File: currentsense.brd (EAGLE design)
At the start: 78.7 x 70.8 mm, 18 parts

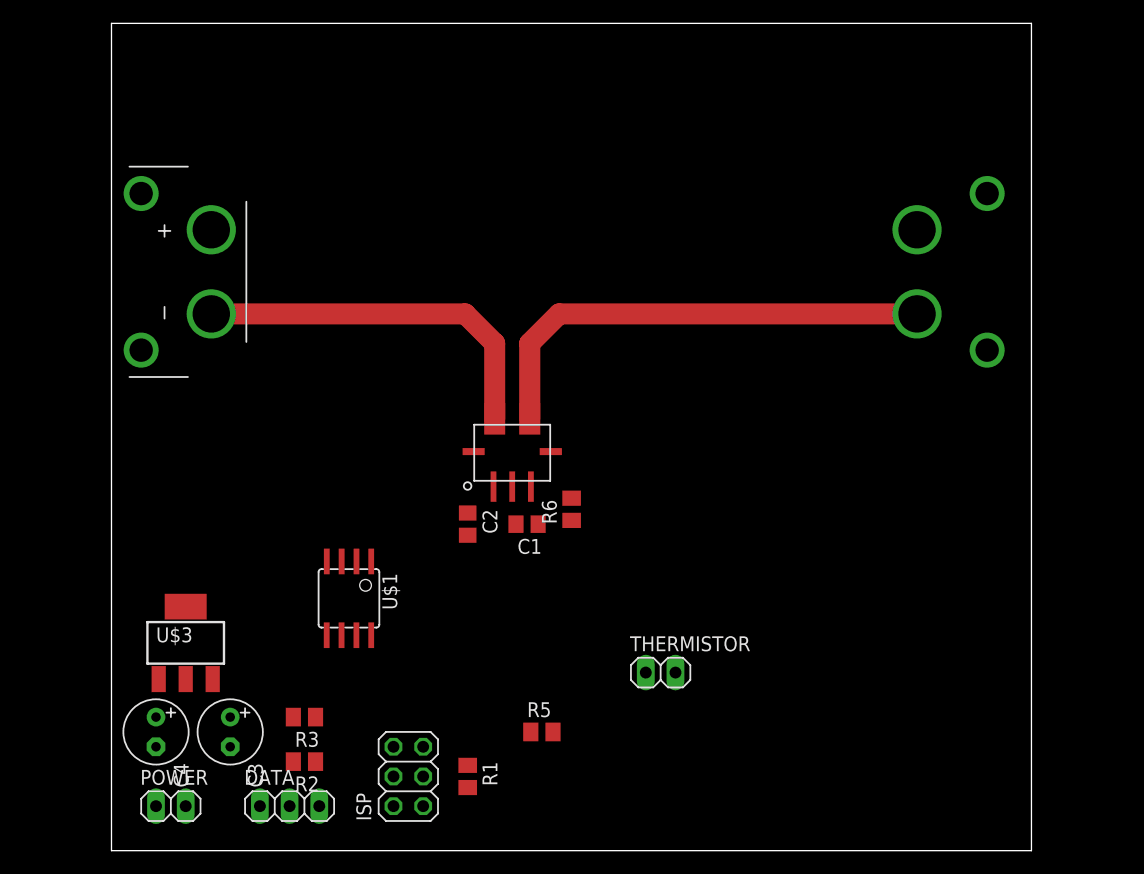
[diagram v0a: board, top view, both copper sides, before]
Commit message: more layout work
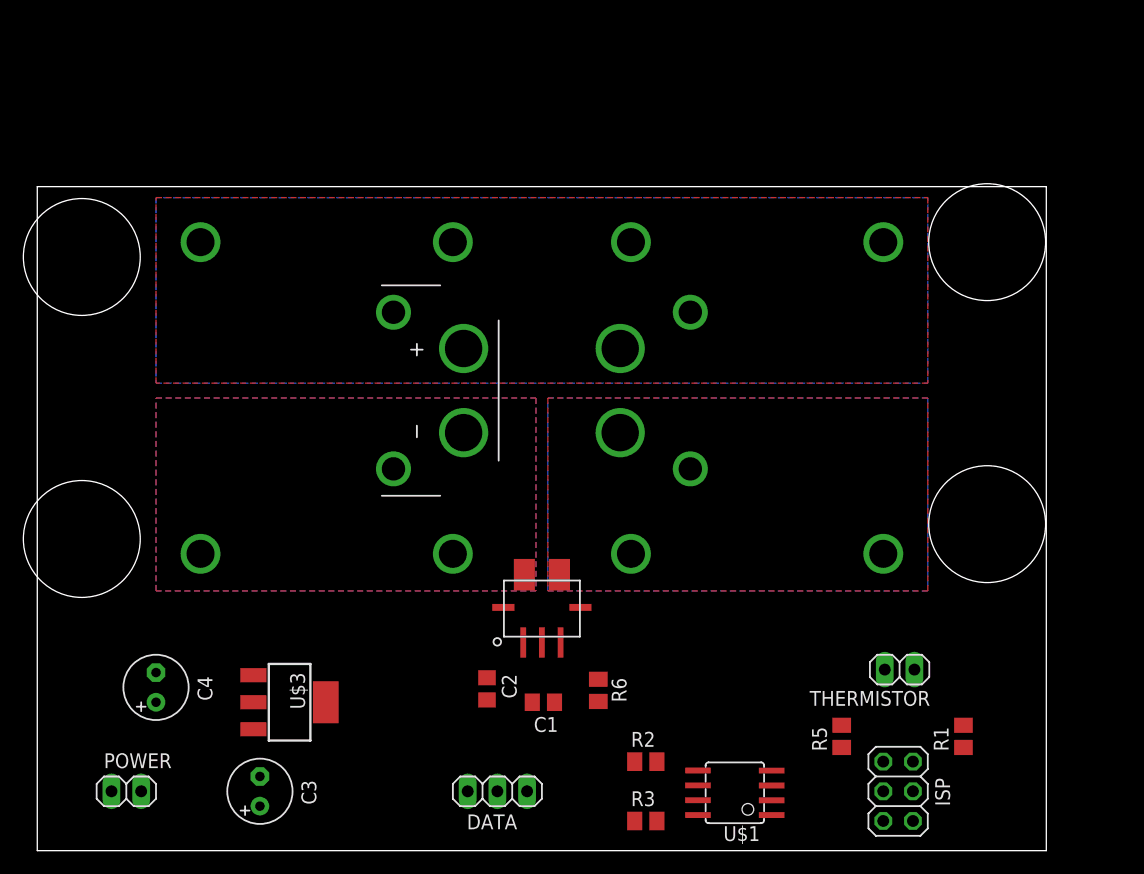
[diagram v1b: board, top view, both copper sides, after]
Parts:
- moved R1 42.6 mm to (72.9, 9.78), turned to 90 degrees
- moved ISP 41.9 mm to (67.3, 5.08)
- moved U$1 37.0 mm to (53.3, 4.95), turned to 90 degrees
- moved R3 30.5 mm to (45.7, 2.54), turned to 0 degrees
- moved R2 29.2 mm to (45.7, 7.62), turned to 0 degrees
- moved U$4 27.4 mm to (49.5, 39.4)
- moved R5 25.7 mm to (62.5, 9.78), turned to 90 degrees
- moved U$5 23.9 mm to (24.1, 39.4)
- moved THERMISTOR 20.4 mm to (67.4, 15.5), turned to 180 degrees
- moved DATA 17.8 mm to (33.0, 5.08)
- moved R6 15.7 mm to (41.7, 13.7)
- moved C1 15.3 mm to (37.0, 12.7)
- moved C2 14.2 mm to (32.1, 13.8)
- moved U$2 13.6 mm to (36.8, 18.4)
- moved U$3 10.2 mm to (15.2, 12.7), turned to 270 degrees
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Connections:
- net N$1 renamed M-IP+
- net N$3 renamed M-IP-
- net N$4 renamed M+
- removed net OC_DETECT: DATA.3
- removed net SDA: DATA.1
- net OC_DETECT/6: now also DATA.2
- net SCL/7: now also DATA.3; no longer DATA.2
- net SDA/5: now also DATA.1
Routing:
- net M-IP+: track 40.6 -> 0.00 mm, vias 0 -> 2
- net M-IP-: track 31.8 -> 0.00 mm, vias 0 -> 2
- added copper zone on layer 1, net M+
- added copper zone on layer 16, net M+
- added copper zone on layer 1, net M-IP+
- added copper zone on layer 16, net M-IP+
- added copper zone on layer 1, net M-IP-
- added copper zone on layer 16, net M-IP-
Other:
- board size 78.7 x 70.8 mm -> 86.3 x 56.8 mm

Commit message: add board files
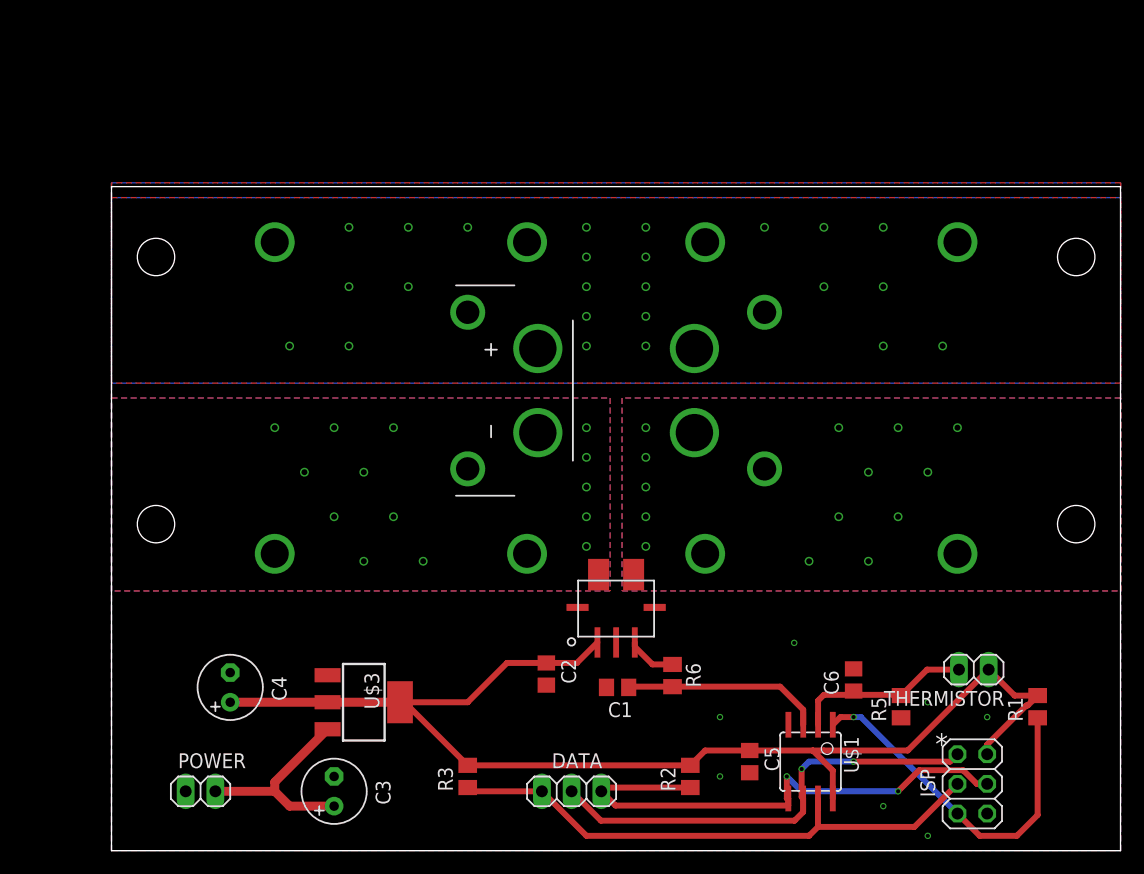
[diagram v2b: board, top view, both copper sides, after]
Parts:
- added C5, C6: 0.1uF, rcl:C0805
- C1, C2: value (none) -> 0.1uF
- C3, C4: value (none) -> 10uF
- R2, R3: value (none) -> 10k
- R6: value (none) -> 2.2k
- moved R3 15.7 mm to (30.5, 6.35), turned to 90 degrees
- moved U$1 7.00 mm to (59.8, 7.62), turned to 180 degrees
- moved R1 6.84 mm to (79.2, 12.3)
- moved C1 6.48 mm to (43.3, 14.0)
- moved R6 6.48 mm to (48.0, 15.0)
- moved ISP 6.38 mm to (73.7, 5.71), turned to 270 degrees
- moved THERMISTOR 6.35 mm to (73.8, 15.5)
- moved C3 6.35 mm to (19.1, 5.08)
- moved U$2 6.35 mm to (43.2, 18.4)
- moved U$4 6.35 mm to (55.9, 39.4)
- moved U$5 6.35 mm to (30.5, 39.4)
- moved C4 6.35 mm to (10.2, 14.0)
- moved POWER 6.35 mm to (7.62, 5.08)
- moved U$3 6.35 mm to (21.6, 12.7)
- moved DATA 6.35 mm to (39.4, 5.08), turned to 180 degrees
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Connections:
- net +3V3: now also C5.1
- net CURRENT: now also U$1.3; no longer U$1.2
- net GND: now also C5.2, C6.2
- net TEMPERATURE: now also C6.1, U$1.2; no longer U$1.3
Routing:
- net +3V3: track 0.00 -> 105.9 mm
- net SCL/7: track 0.00 -> 47.9 mm
- net SDA/5: track 0.00 -> 45.8 mm, vias 0 -> 2
- net OC_DETECT/6: track 0.00 -> 38.8 mm, vias 0 -> 2
- net RESET: track 0.00 -> 31.1 mm, vias 0 -> 1
- net VCC: track 0.00 -> 17.9 mm
- net CURRENT: track 0.00 -> 17.1 mm
- net TEMPERATURE: track 0.00 -> 15.3 mm
- net N$2: track 0.00 -> 4.22 mm
- added copper zone on layer 1, net GND
- added copper zone on layer 16, net GND
- added copper zone on layer 15, net M+
- added copper zone on layer 2, net M+
- added copper zone on layer 15, net M-IP+
- added copper zone on layer 2, net M-IP+
- added copper zone on layer 15, net M-IP-
- added copper zone on layer 2, net M-IP-
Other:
- board text added: "*"
